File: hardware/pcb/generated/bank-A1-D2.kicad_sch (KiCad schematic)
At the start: 34 parts, among them U1 TCA9554DWR, U18 SK9822-EC20, U19 SK9822-EC20, U20 SK9822-EC20, U21 SK9822-EC20, U6 SK9822-EC20, U7 SK9822-EC20, U8 SK9822-EC20, U9 SK9822-EC20

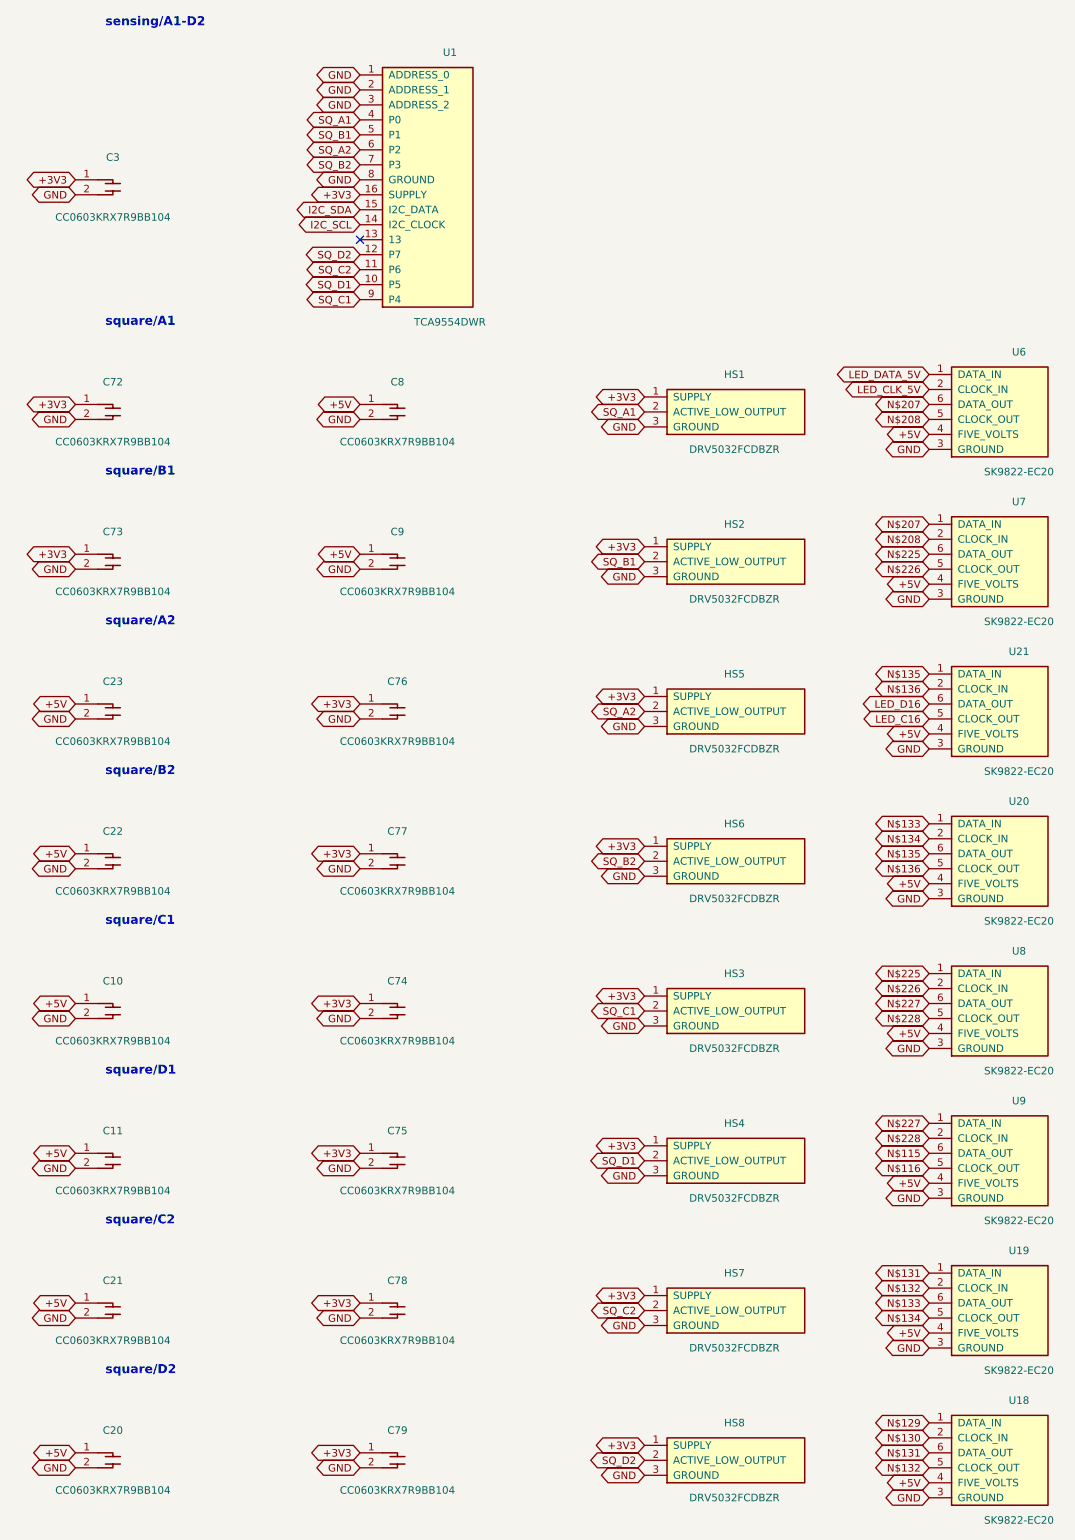
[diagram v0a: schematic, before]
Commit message: chore(pcb): regenerate KiCad, SPICE and review output
Generated by `just pcb` from the committed definition; not hand-edited.
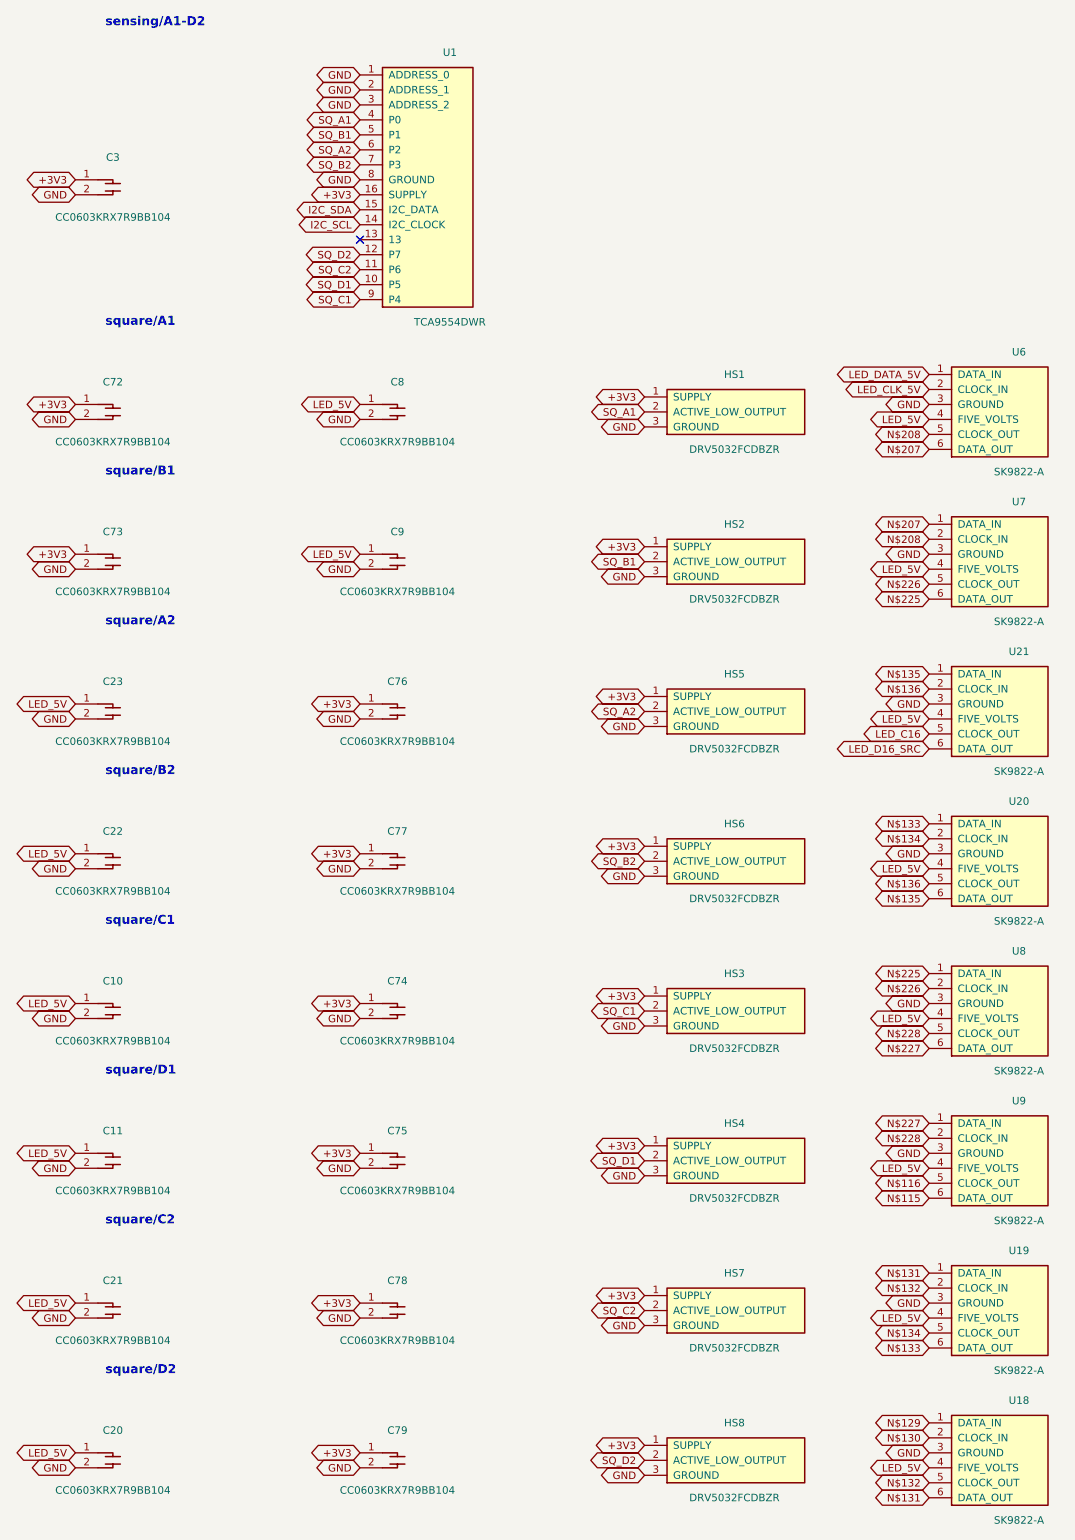
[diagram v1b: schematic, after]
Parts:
- U18, U19, U20, U21, U6, U7, U8, U9: value SK9822-EC20 -> SK9822-A
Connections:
- net +5V renamed LED_5V
- net LED_D16 renamed LED_D16_SRC
